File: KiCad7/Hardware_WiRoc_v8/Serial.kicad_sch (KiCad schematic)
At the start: 7 parts, among them J4 Conn_01x09_Socket, U8 SP3232ECY-L

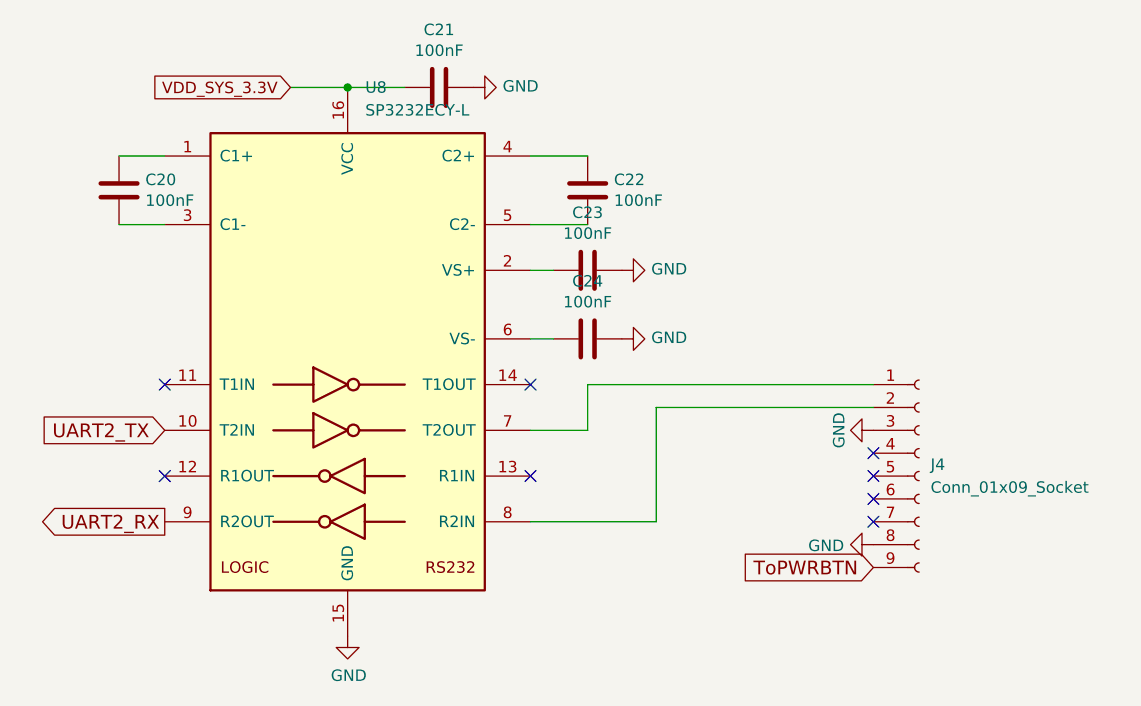
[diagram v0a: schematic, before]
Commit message: sbc version etc
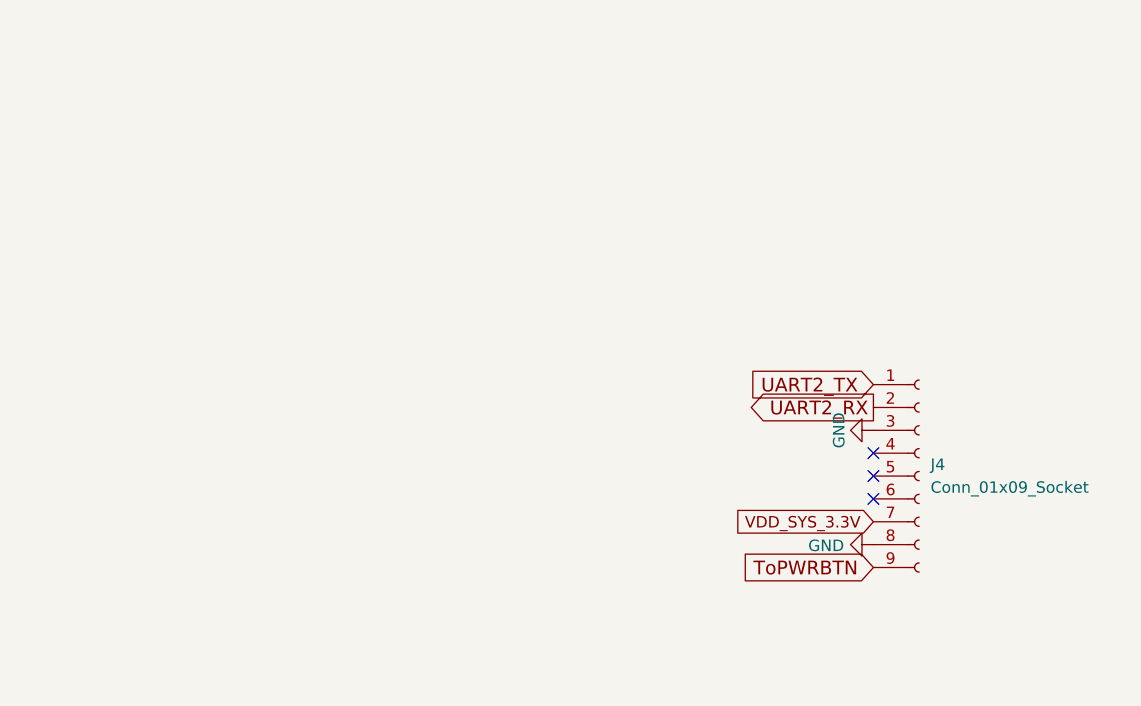
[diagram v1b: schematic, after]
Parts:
- removed C20, C21, C22, C23, C24: 100nF, Capacitor_SMD:C_0603_1608Metric, symbol Device:C
- removed U8: SP3232ECY-L, Package_SO:TSSOP-16_4.4x5mm_P0.65mm, symbol Interface_UART:MAX3232
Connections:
- net UART2_RX: now also J4.2 (Pin_2)
- net UART2_TX: now also J4.1 (Pin_1)
- net VDD_SYS_3.3V: now also J4.7 (Pin_7)
- no-connect marks 8 -> 3
